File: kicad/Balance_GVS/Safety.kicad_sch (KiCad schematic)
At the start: 25 parts, among them J1 Conn_01x02_Pin, K1 AQY210S, Q3 2N3904, Q4 2N3904, SW2 EVQ-P7A01P, U3 OPA4313IPWR, U4 INA303A1IPW

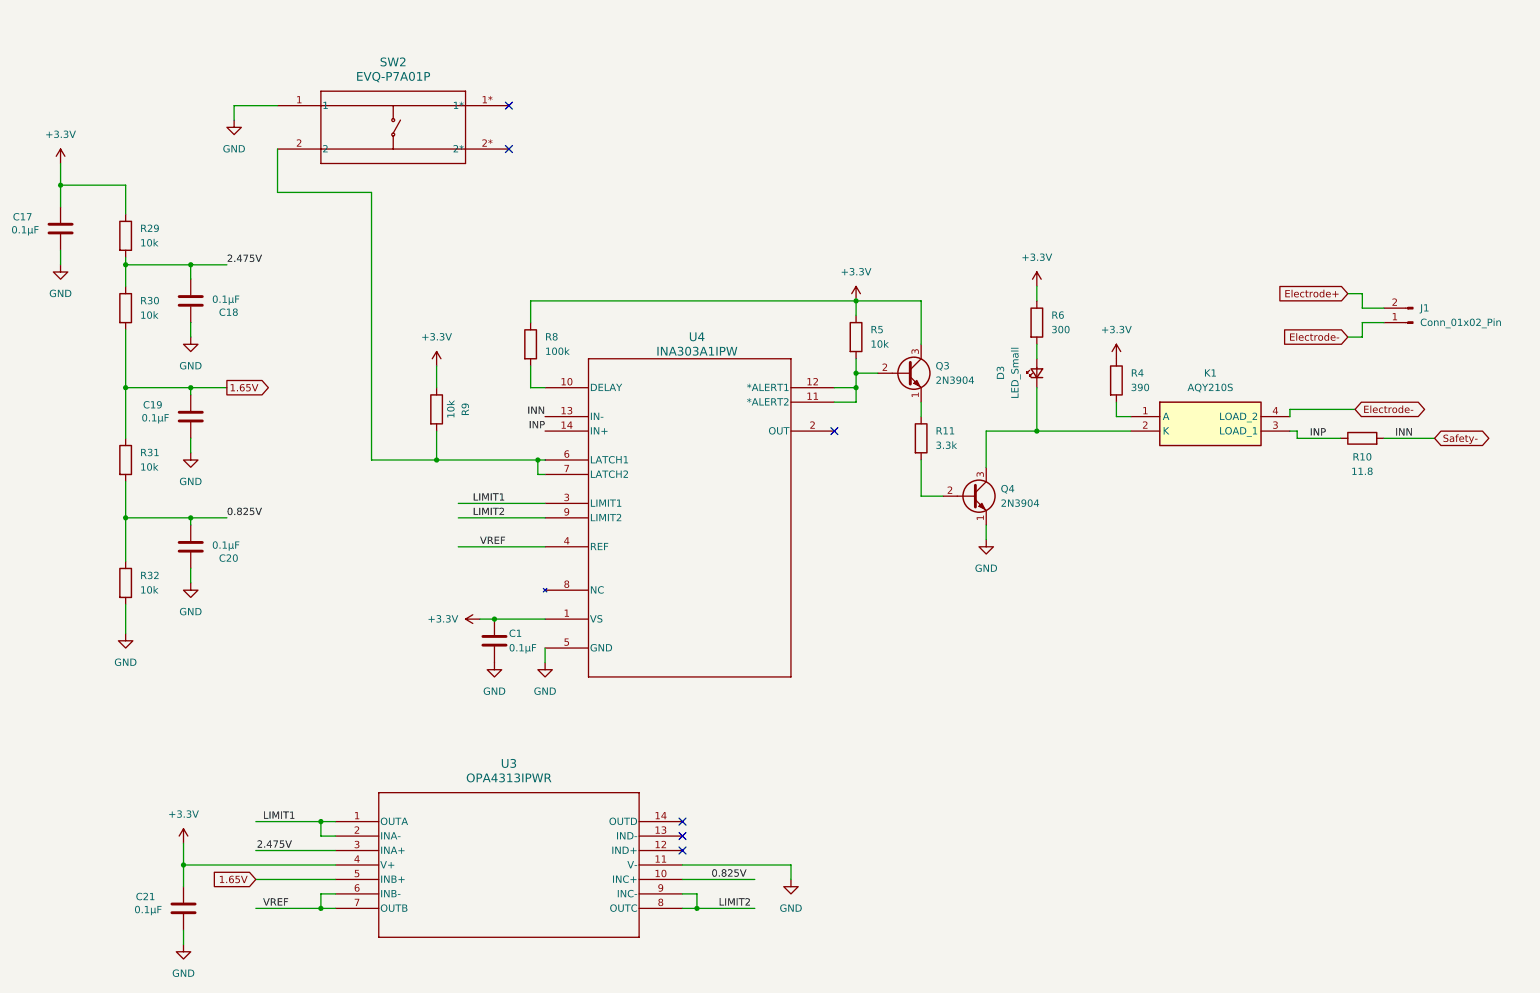
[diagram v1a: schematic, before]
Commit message: Add shit ton to schematic
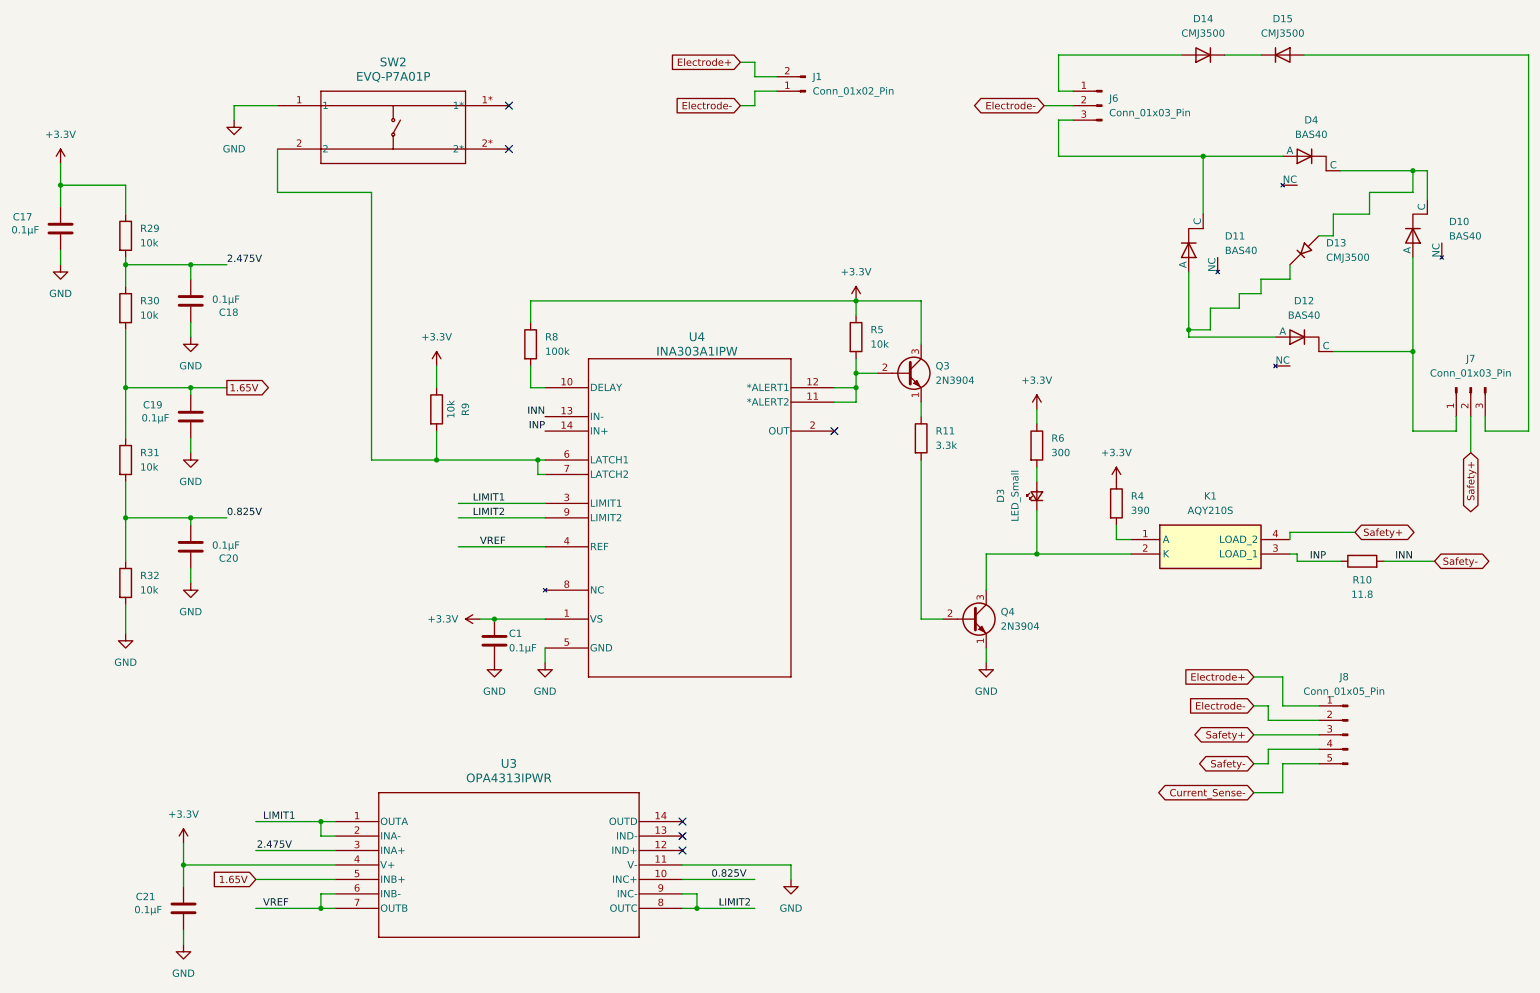
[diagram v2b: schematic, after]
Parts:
- added D10, D11, D12, D4: BAS40, BAS40:P200_SOT-23, symbol BAS40:Diode-NC_pin
- added D13: CMJ3500, Diode_SMD:D_SOD-123F, symbol Device:D_45deg
- added D14, D15: CMJ3500, Diode_SMD:D_SOD-123F, symbol Device:D
- added J6, J7: Conn_01x03_Pin, Connector_PinHeader_2.54mm:PinHeader_1x03_P2.54mm_Vertical, symbol Connector:Conn_01x03_Pin
- added J8: Conn_01x05_Pin, Connector_PinSocket_2.54mm:PinSocket_1x05_P2.54mm_Vertical, symbol Connector:Conn_01x05_Pin
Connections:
- net Electrode+: now also J8.1 (Pin_1)
- net Electrode-: now also J6.2 (Pin_2), J8.2 (Pin_2); no longer K1.4 (LOAD_2)
- net Safety-: now also J8.4 (Pin_4)
- new net: D11.1 (A), D12.1 (A), D13.1 (K)
- new net: D10.1 (A), D12.2 (C), J7.1 (Pin_1)
- new net: D10.2 (C), D13.2 (A), D4.2 (C)
- new net: D14.1 (K), D15.1 (K)
- new net: D15.2 (A), J7.3 (Pin_3)
- new net: D14.2 (A), J6.1 (Pin_1)
- new net: D11.2 (C), D4.1 (A), J6.3 (Pin_3)
- new net Current_Sense-: J8.5 (Pin_5)
- new net Safety+: J7.2 (Pin_2), J8.3 (Pin_3), K1.4 (LOAD_2)
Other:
- moved on the sheet: D3, J1, K1, Q4, R10, R4, R6
